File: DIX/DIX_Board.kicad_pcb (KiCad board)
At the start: 2 copper layers, 34 parts, among them J1 Conn_01x12_Male, J2 Conn_01x12_Male, U1 AMS1117-3.3, U3 TPS79318-EP

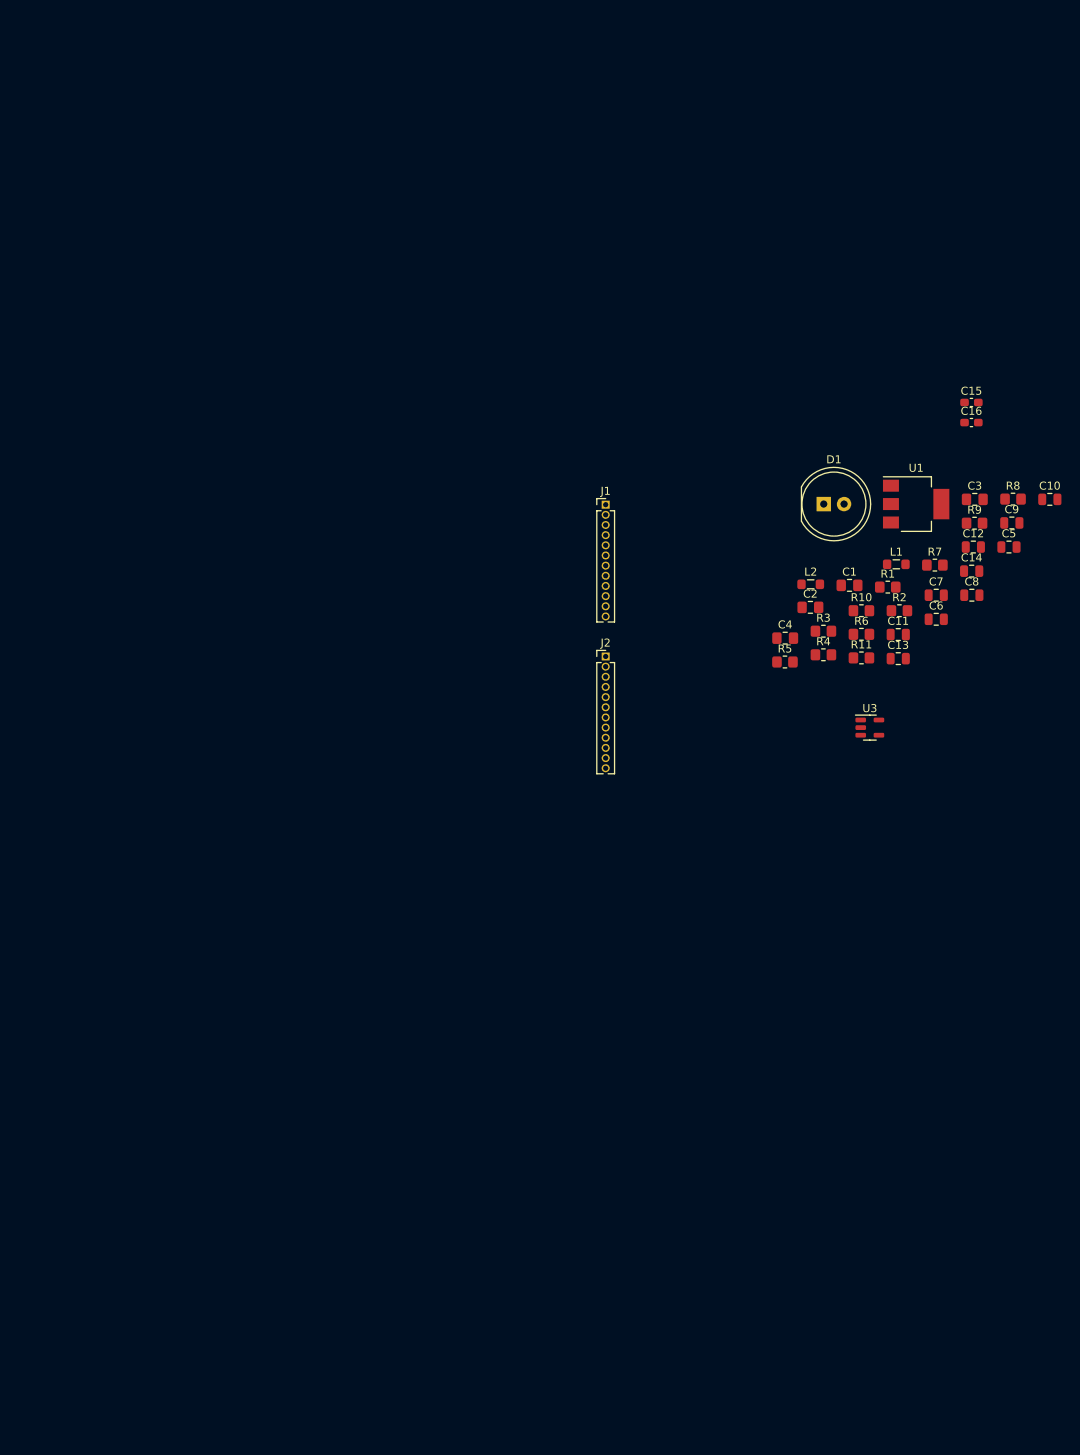
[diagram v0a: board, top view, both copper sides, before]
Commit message: Some routing
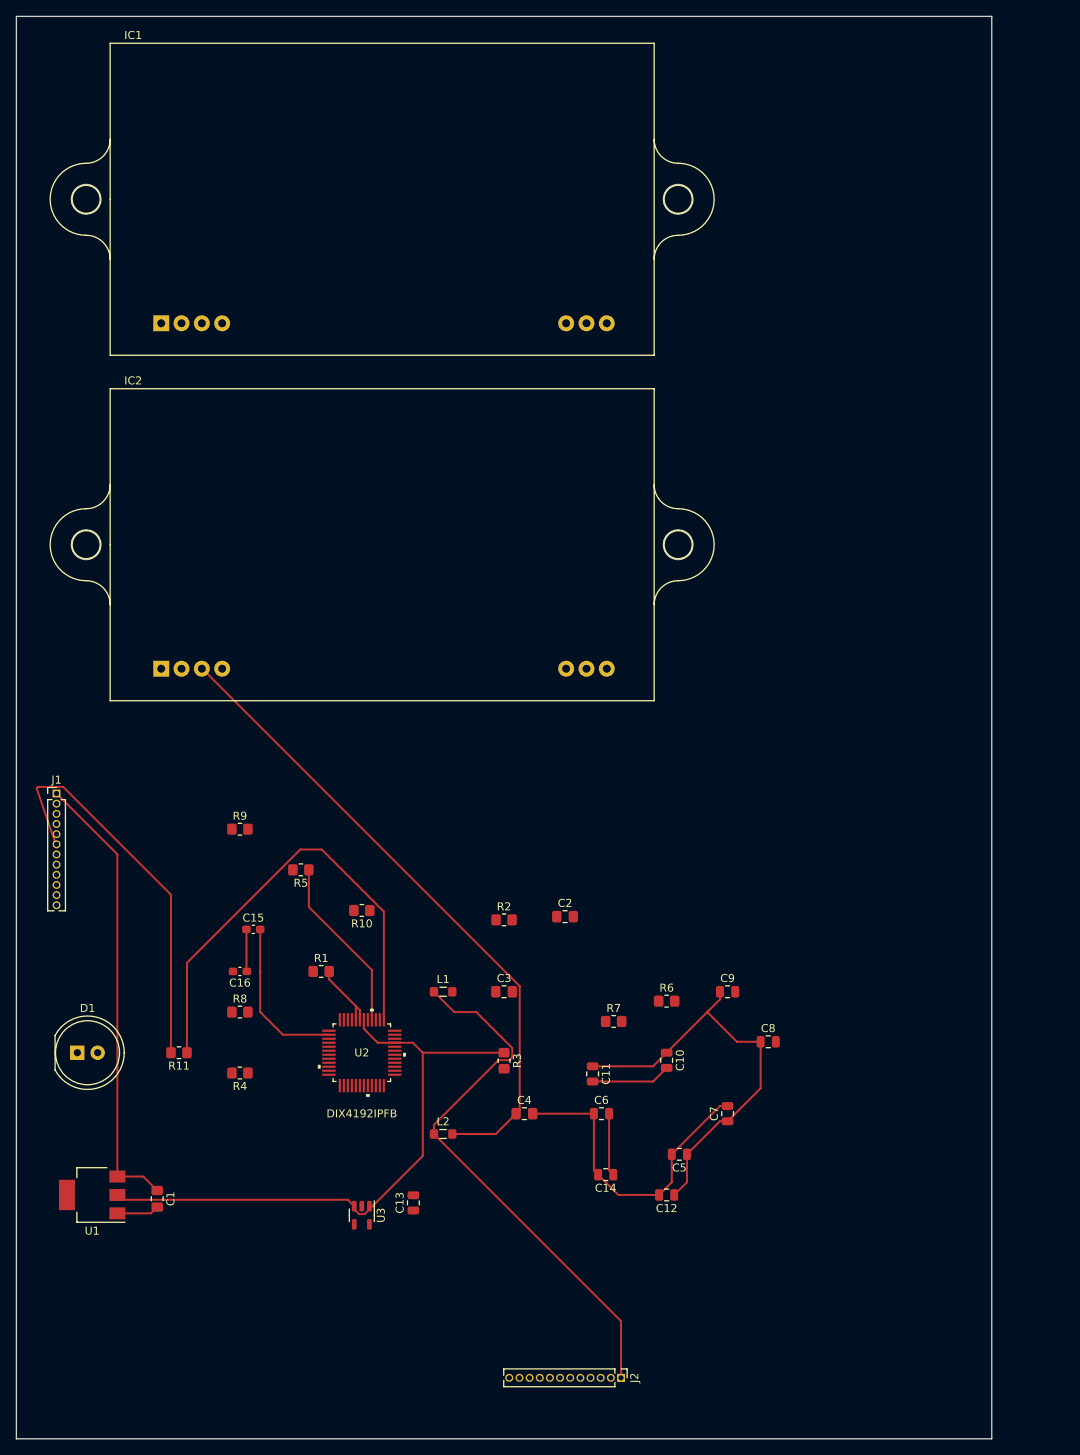
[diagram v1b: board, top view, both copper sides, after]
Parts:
- added IC1: TORX1950A_F_, Audio_Module:Reverb_BTDR-1H, F.Cu at (48.6, 53.6)
- added IC2: TORX1950A_F_, Audio_Module:Reverb_BTDR-1H, F.Cu at (48.6, 96.8)
- added U2: DIX4192IPFB, DIX Footprints:DIX4192IPFB, F.Cu at (73.7, 144.8)
- moved U1 134.4 mm to (40.0, 162.6), turned to 180 degrees
- moved R8 116.0 mm to (58.4, 139.7)
- moved D1 115.8 mm to (38.1, 144.8)
- moved C1 115.6 mm to (48.1, 163.0), turned to -90 degrees
- moved C16 114.3 mm to (58.4, 134.6), turned to 180 degrees
- moved C15 111.3 mm to (60.1, 129.4)
- moved R9 99.5 mm to (58.4, 116.8)
- moved R11 98.6 mm to (50.8, 144.8), turned to 180 degrees
- moved C13 91.1 mm to (80.1, 163.5), turned to 90 degrees
- moved J2 90.2 mm to (106.1, 185.4), turned to -90 degrees
- moved R4 89.7 mm to (58.4, 147.3), turned to 180 degrees
- moved C12 89.6 mm to (111.8, 162.6), turned to 180 degrees
- moved C14 88.2 mm to (104.1, 160.0), turned to 180 degrees
- moved U3 88.0 mm to (73.7, 165.1), turned to -90 degrees
- moved C5 86.4 mm to (113.3, 157.5), turned to 180 degrees
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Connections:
- J1 pad 10: unconnected-(J1-Pad10) -> SDOUTB
- J1 pad 2: unconnected-(J1-Pad2) -> MCLK
- J1 pad 3: unconnected-(J1-Pad3) -> BCKA
- J1 pad 4: unconnected-(J1-Pad4) -> LRCKA
- J1 pad 5: unconnected-(J1-Pad5) -> SDINA
- J1 pad 6: unconnected-(J1-Pad6) -> SDOUTA
- J1 pad 7: unconnected-(J1-Pad7) -> BCKB
- J1 pad 8: unconnected-(J1-Pad8) -> LRCKB
- J1 pad 9: unconnected-(J1-Pad9) -> SDINB
- J2 pad 1: MCLK -> +5V
- J2 pad 10: unconnected-(J2-Pad10) -> CCLK/SCL
- J2 pad 11: unconnected-(J2-Pad11) -> *CS/AO
- J2 pad 12: unconnected-(J2-Pad12) -> CPM
- J2 pad 2: unconnected-(J2-Pad2) -> TX+
- J2 pad 3: unconnected-(J2-Pad3) -> TX-
- J2 pad 4: unconnected-(J2-Pad4) -> GPO4
- J2 pad 5: unconnected-(J2-Pad5) -> GPO3
- J2 pad 6: unconnected-(J2-Pad6) -> GPO2
- J2 pad 7: unconnected-(J2-Pad7) -> GPO1
- J2 pad 8: unconnected-(J2-Pad8) -> CDOUT/SDA
- J2 pad 9: unconnected-(J2-Pad9) -> CDIN/A1
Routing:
- net +3.3V: track 0.00 -> 127.9 mm
- net Net-(C4-Pad1): track 0.00 -> 81.3 mm
- net +5V: track 0.00 -> 68.5 mm
- net GND: track 0.00 -> 59.3 mm
- net Net-(R11-Pad1): track 0.00 -> 58.5 mm
- net VBUS: track 0.00 -> 56.7 mm
- net SDOUTA: track 0.00 -> 50.0 mm
- net Net-(R5-Pad1): track 0.00 -> 22.0 mm
- net Net-(C15-Pad2): track 0.00 -> 20.3 mm
- net Net-(C10-Pad2): track 0.00 -> 9.96 mm
- net +1V8: track 0.00 -> 7.84 mm
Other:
- board outline added: 121.9 x 177.8 mm
